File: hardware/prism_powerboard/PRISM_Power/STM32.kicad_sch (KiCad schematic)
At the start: 1 part, among them U1 STM32G031F6Px

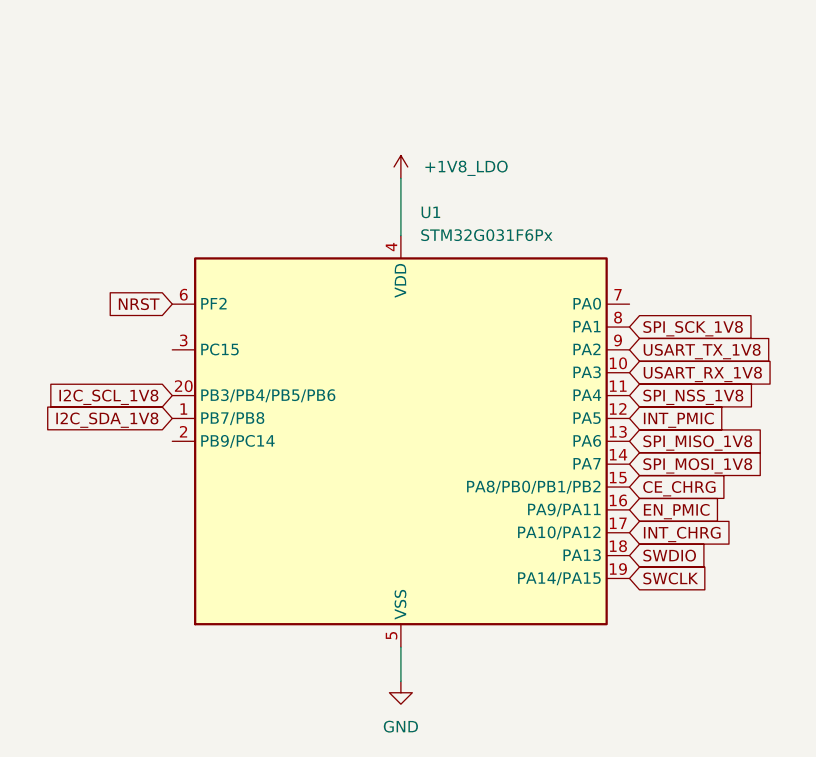
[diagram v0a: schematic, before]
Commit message: DRC Required
Everything should be done, just reviewing DRC and making sure everything looks good. Quite a few errors, few seem to be relevant or real.
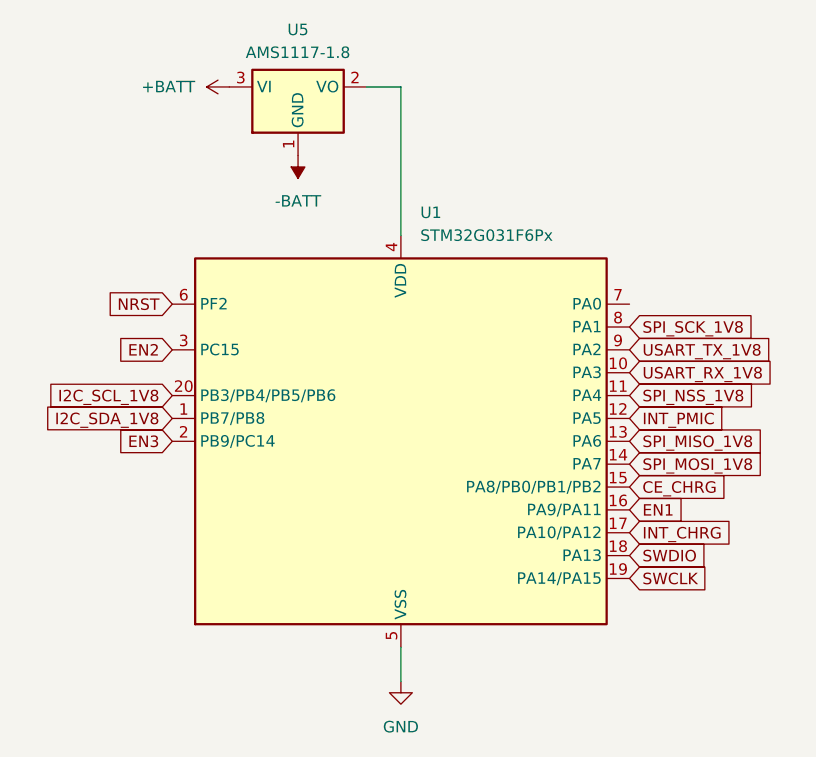
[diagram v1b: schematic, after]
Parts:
- added U5: AMS1117-1.8, Package_TO_SOT_SMD:SOT-223-3_TabPin2, symbol Regulator_Linear:AMS1117-1.8
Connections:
- net EN3: now reaches U1.2 (PB9/PC14)
- net EN2: now reaches U1.3 (PC15)
- net +1V8_LDO: no longer names the net of U1.4 (VDD)
- net +1V8_LDO: now also U5.2 (VO)
- net EN_PMIC renamed EN1
- new net +BATT: U5.3 (VI)
- new net -BATT: U5.1 (GND)
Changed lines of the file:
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@@
+	(wire
+		(pts
+			(xy 137.16 36.83) (xy 140.97 36.83)
+		)
+		(stroke
+			(width 0)
+			(type default)
+		)
+	)
 	(wire
 		(pts
@@
 	(wire
 		(pts
-			(xy 140.97 46.99) (xy 140.97 53.34)
+			(xy 140.97 36.83) (xy 140.97 53.34)
 		)
 		(stroke
@@
 		)
 	)
+	(global_label "EN3"
+		(shape input)
+		(at 115.57 76.2 180)
+		(fields_autoplaced yes)
+		(effects
+			(font
+				(size 1.27 1.27)
+			)
+			(justify right)
+		)
+		(property "Intersheetrefs" "${INTERSHEET_REFS}"
+			(at 108.8958 76.2 0)
+			(hide yes)
+			(show_name no)
+			(do_not_autoplace no)
+			(effects
+				(font
+					(size 1.27 1.27)
+				)
+				(justify right)
+			)
+		)
+	)
 	(global_label "USART_TX_1V8"
 		(shape input)
@@
 		)
 	)
+	(global_label "EN2"
+		(shape input)
+		(at 115.57 66.04 180)
+		(fields_autoplaced yes)
+		(effects
+			(font
+				(size 1.27 1.27)
+			)
+			(justify right)
+		)
+		(property "Intersheetrefs" "${INTERSHEET_REFS}"
+			(at 108.8958 66.04 0)
+			(hide yes)
+			(show_name no)
+			(do_not_autoplace no)
+			(effects
+				(font
+					(size 1.27 1.27)
+				)
+				(justify right)
+			)
+		)
+	)
 	(global_label "SPI_SCK_1V8"
 		(shape input)
@@
 		)
 	)
-	(global_label "EN_PMIC"
+	(global_label "EN1"
 		(shape input)
 		(at 166.37 83.82 0)
@@
 		)
 		(property "Intersheetrefs" "${INTERSHEET_REFS}"
-			(at 177.3985 83.82 0)
+			(at 173.0442 83.82 0)
 			(hide yes)
 			(show_name no)
@@
 	)
 	(symbol
-		(lib_id "power:+1V8")
-		(at 140.97 46.99 0)
+		(lib_id "power:-BATT")
+		(at 129.54 44.45 180)
 		(unit 1)
 		(body_style 1)
@@
 		(dnp no)
 		(fields_autoplaced yes)
+		(property "Reference" "#PWR045"
+			(at 129.54 40.64 0)
+			(hide yes)
+			(show_name no)
+			(do_not_autoplace no)
+			(effects
+				(font
+					(size 1.27 1.27)
+				)
+			)
+		)
+		(property "Value" "-BATT"
+			(at 129.54 49.53 0)
+			(show_name no)
+			(do_not_autoplace no)
+			(effects
+				(font
+					(size 1.27 1.27)
+				)
+			)
+		)
+		(property "Footprint" ""
+			(at 129.54 44.45 0)
+			(hide yes)
+			(show_name no)
+			(do_not_autoplace no)
+			(effects
+				(font
+					(size 1.27 1.27)
+				)
+			)
+		)
+		(property "Datasheet" ""
+			(at 129.54 44.45 0)
+			(hide yes)
+			(show_name no)
+			(do_not_autoplace no)
+			(effects
+				(font
+					(size 1.27 1.27)
+				)
+			)
+		)
+		(property "Description" "Power symbol creates a global label with name \"-BATT\""
+			(at 129.54 44.45 0)
+			(hide yes)
+			(show_name no)
+			(do_not_autoplace no)
+			(effects
+				(font
+					(size 1.27 1.27)
+				)
+			)
+		)
+		(pin "1"
+		)
+		(instances
+			(project "PRISM_Power"
+				(path "/80548bcf-507c-4ded-a0d2-b94774a2c706/b034b59f-81b0-4395-9c56-0258adc1e6aa"
+					(reference "#PWR045")
+					(unit 1)
+				)
+			)
+		)
+	)
+	(symbol
+		(lib_id "Regulator_Linear:AMS1117-1.8")
+		(at 129.54 36.83 0)
+		(unit 1)
+		(body_style 1)
+		(exclude_from_sim no)
+		(in_bom yes)
+		(on_board yes)
+		(in_pos_files yes)
+		(dnp no)
+		(fields_autoplaced yes)
+		(property "Reference" "U5"
+			(at 129.54 30.48 0)
+			(show_name no)
+			(do_not_autoplace no)
+			(effects
+				(font
+					(size 1.27 1.27)
+				)
+			)
+		)
+		(property "Value" "AMS1117-1.8"
+			(at 129.54 33.02 0)
+			(show_name no)
+			(do_not_autoplace no)
+			(effects
+				(font
+					(size 1.27 1.27)
+				)
+			)
+		)
+		(property "Footprint" "Package_TO_SOT_SMD:SOT-223-3_TabPin2"
+			(at 129.54 31.75 0)
+			(hide yes)
+			(show_name no)
+			(do_not_autoplace no)
+			(effects
+				(font
+					(size 1.27 1.27)
+				)
+			)
+		)
+		(property "Datasheet" "http://www.advanced-monolithic.com/pdf/ds1117.pdf"
+			(at 132.08 43.18 0)
+			(hide yes)
+			(show_name no)
+			(do_not_autoplace no)
+			(effects
+				(font
+					(size 1.27 1.27)
+				)
+			)
+		)
+		(property "Description" "1A Low Dropout regulator, positive, 1.8V fixed output, SOT-223"
+			(at 129.54 36.83 0)
+			(hide yes)
+			(show_name no)
+			(do_not_autoplace no)
+			(effects
+				(font
+					(size 1.27 1.27)
+				)
+			)
+		)
+		(pin "3"
+		)
+		(pin "2"
+		)
+		(pin "1"
+		)
+		(instances
+			(project "PRISM_Power"
+				(path "/80548bcf-507c-4ded-a0d2-b94774a2c706/b034b59f-81b0-4395-9c56-0258adc1e6aa"
+					(reference "U5")
+					(unit 1)
+				)
+			)
+		)
+	)
+	(symbol
+		(lib_id "power:+BATT")
+		(at 121.92 36.83 90)
+		(unit 1)
+		(body_style 1)
+		(exclude_from_sim no)
+		(in_bom yes)
+		(on_board yes)
+		(in_pos_files yes)
+		(dnp no)
+		(fields_autoplaced yes)
 		(property "Reference" "#PWR06"
-			(at 140.97 50.8 0)
-			(hide yes)
-			(show_name no)
-			(do_not_autoplace no)
-			(effects
-				(font
-					(size 1.27 1.27)
-				)
-			)
-		)
-		(property "Value" "+1V8_LDO"
-			(at 143.51 45.7199 0)
+			(at 125.73 36.83 0)
+			(hide yes)
+			(show_name no)
+			(do_not_autoplace no)
+			(effects
+				(font
+					(size 1.27 1.27)
+				)
+			)
+		)
+		(property "Value" "+BATT"
+			(at 118.11 36.8299 90)
 			(show_name no)
 			(do_not_autoplace no)
@@
 		)
 		(property "Footprint" ""
-			(at 140.97 46.99 0)
+			(at 121.92 36.83 0)
 			(hide yes)
 			(show_name no)
@@
 		)
 		(property "Datasheet" ""
-			(at 140.97 46.99 0)
-			(hide yes)
-			(show_name no)
-			(do_not_autoplace no)
-			(effects
-				(font
-					(size 1.27 1.27)
-				)
-			)
-		)
-		(property "Description" "Power symbol creates a global label with name \"+1V8\""
-			(at 140.97 46.99 0)
-			(hide yes)
-			(show_name no)
+			(at 121.92 36.83 0)
+			(hide yes)
+			(show_name no)
+			(do_not_autoplace no)
+			(effects
+				(font
+					(size 1.27 1.27)
+				)
+			)
+		)
+		(property "Description" "Power symbol creates a global label with name \"+BATT\""
+			(at 121.92 36.83 0)
+			(hide yes)
+			(show_name no)
